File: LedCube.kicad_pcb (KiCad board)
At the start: 2 copper layers, 102 x 102 mm, 37 parts, among them J12 B10B-PHDSS-B_LF__SN_, J13 B10B-PHDSS-B_LF__SN_, J14 B10B-PHDSS-B_LF__SN_, J15 B10B-PHDSS-B_LF__SN_, J16 B10B-PHDSS-B_LF__SN_, J17 B10B-PHDSS-B_LF__SN_, J18 B10B-PHDSS-B_LF__SN_, J19 B10B-PHDSS-B_LF__SN_, J20 B10B-PHDSS-B_LF__SN_, J21 B10B-PHDSS-B_LF__SN_, U1 STM32H743VGTx, U10 SN74LVC373ARGYR, U11 SN74LVC373ARGYR, U12 SN74LVC373ARGYR, U13 SN74LVC373ARGYR, U14 SN74LVC373ARGYR, U2 SN74LVC373ARGYR, U3 SN74LVC373ARGYR, U4 SN74LVC373ARGYR, U5 SN74LVC373ARGYR, U6 SN74LVC373ARGYR, U7 SN74LVC373ARGYR, U8 SN74LVC373ARGYR, U9 SN74LVC373ARGYR

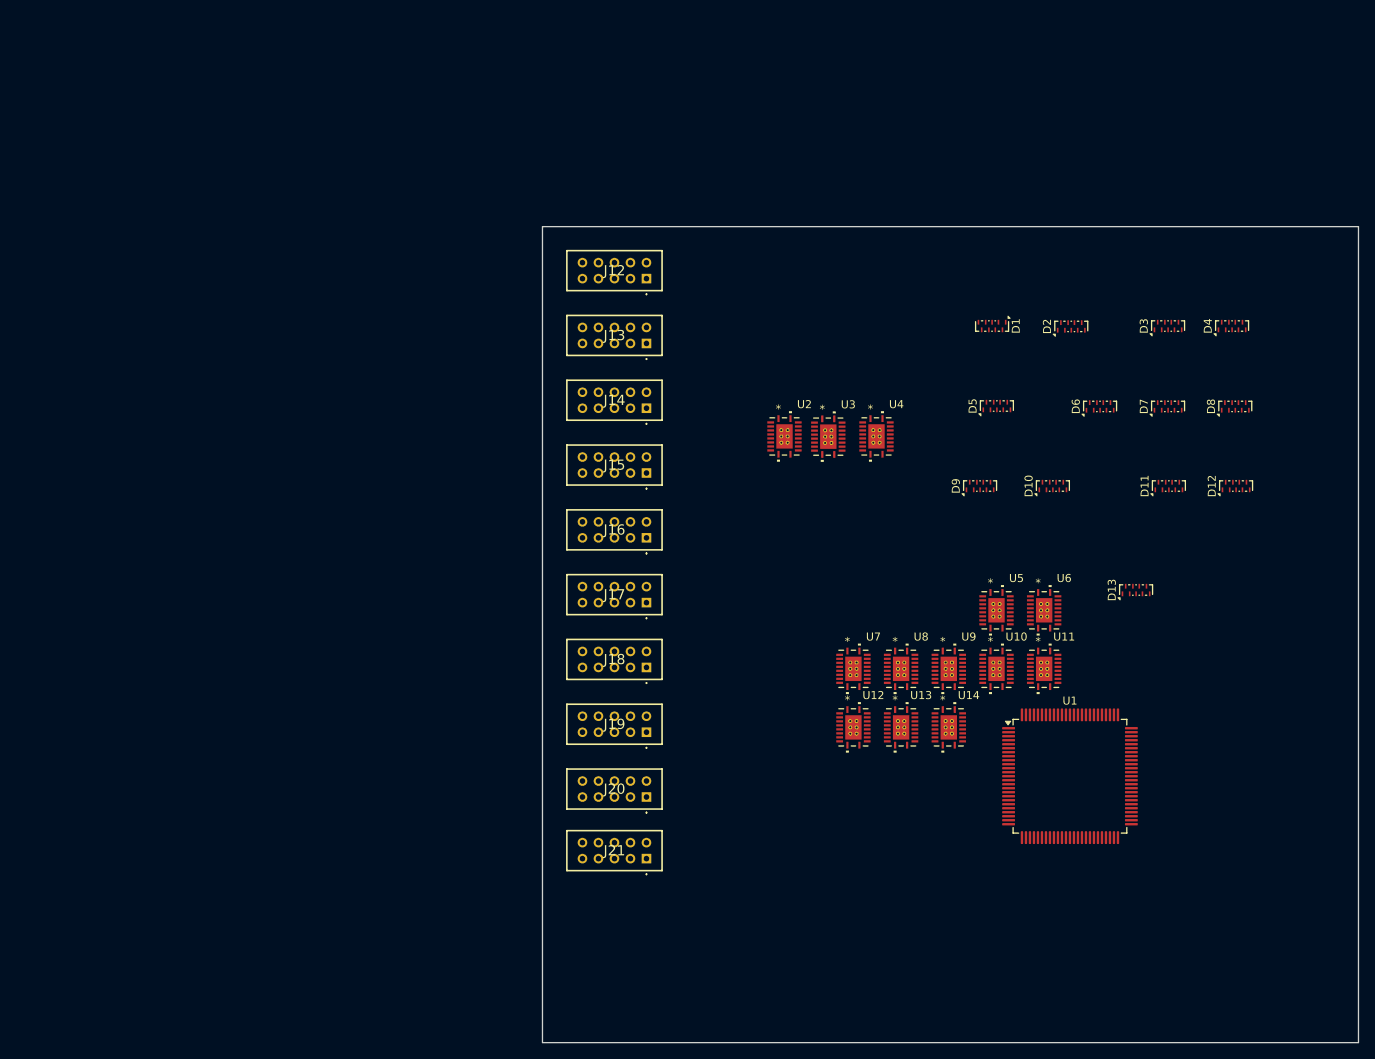
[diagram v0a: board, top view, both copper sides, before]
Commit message: Schematic + PCB
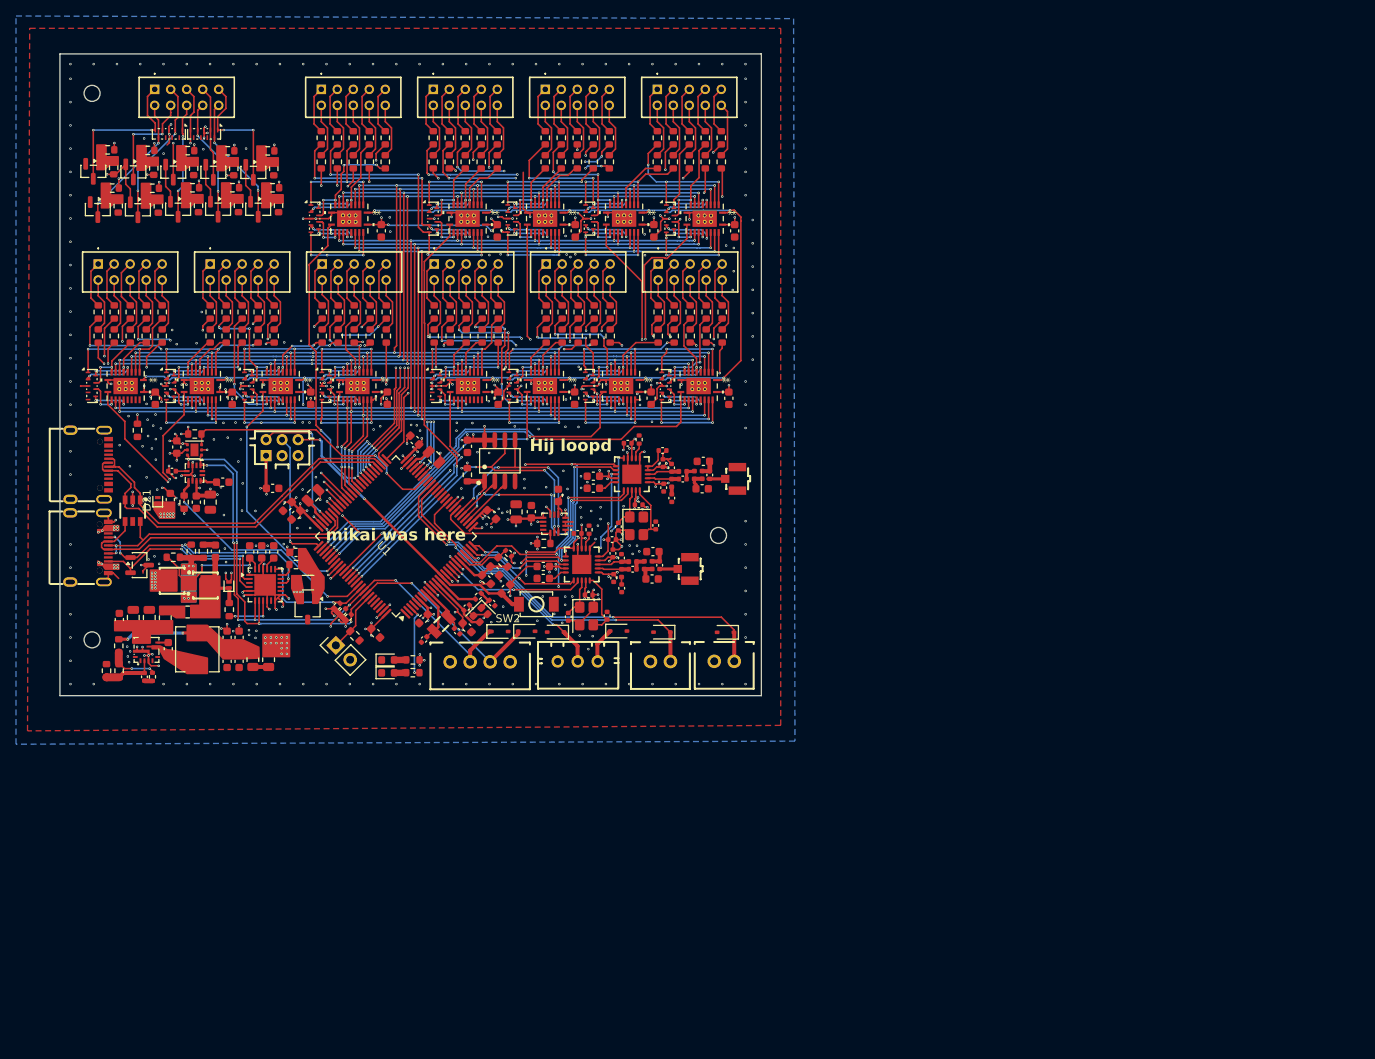
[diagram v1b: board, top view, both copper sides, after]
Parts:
- removed J12, J13, J14, J15, J16, J17, J18, J19, J20, J21: B10B-PHDSS-B_LF__SN_, JST B10B-PHDSS-B(LF)(SN):B10BPHDSSBLFSN
- added C1: 100nF, Capacitor_SMD:C_0603_1608Metric, F.Cu at (89.4, 100.8)
- added C10: 100nF, Capacitor_SMD:C_0603_1608Metric, F.Cu at (84.6, 105.6)
- added C11: 2.2uF, < 100mΩ, Capacitor_SMD:C_0805_2012Metric, F.Cu at (80.4, 84.3)
- added C12: 100nF, Capacitor_SMD:C_0603_1608Metric, F.Cu at (79.1, 104.5)
- added C13: 2.2uF, < 100mΩ, Capacitor_SMD:C_0805_2012Metric, F.Cu at (65.3, 89.1)
- added C14: 4.7uF, Capacitor_SMD:C_0603_1608Metric, F.Cu at (62.1, 90.5)
- added C17: 15pF, Capacitor_SMD:C_0402_1005Metric, F.Cu at (79.2, 107.1)
- added C18: 15pF, Capacitor_SMD:C_0402_1005Metric, F.Cu at (83.3, 106.1)
- added C19: 100nF, Capacitor_SMD:C_0603_1608Metric, F.Cu at (84.6, 83.0)
- added C2: 1uF, Capacitor_SMD:C_0603_1608Metric, F.Cu at (87.0, 99.6)
- added C20: 100nF, Capacitor_SMD:C_0603_1608Metric, F.Cu at (60.3, 88.2)
- added C21: 10uF, Capacitor_SMD:C_0805_2012Metric, F.Cu at (44.9, 104.4)
- added C22: 10uF, Capacitor_SMD:C_0805_2012Metric, F.Cu at (42.9, 104.4)
- added C23: 100nF, Capacitor_SMD:C_0603_1608Metric, F.Cu at (41.1, 104.6)
- added C24: 100nF, Capacitor_SMD:C_0603_1608Metric, F.Cu at (47.2, 108.3)
- added C25: 100pF, Capacitor_SMD:C_0402_1005Metric, F.Cu at (44.2, 111.8)
- added C26: 22uF, Capacitor_SMD:C_0603_1608Metric, F.Cu at (54.6, 106.8)
- added C27: 22uF, Capacitor_SMD:C_0603_1608Metric, F.Cu at (56.1, 106.8)
- added C28: 22uF, Capacitor_SMD:C_0603_1608Metric, F.Cu at (54.6, 109.8)
- added C29: 100nF, Capacitor_SMD:C_0603_1608Metric, F.Cu at (56.1, 109.8)
- added C3: 100nF, Capacitor_SMD:C_0603_1608Metric, F.Cu at (88.0, 98.5)
- added C30: 100nF, Capacitor_SMD:C_0603_1608Metric, F.Cu at (117.3, 77.0)
- added C31: 100nF, Capacitor_SMD:C_0603_1608Metric, F.Cu at (74.6, 76.9)
- added C32: 100nF, Capacitor_SMD:C_0603_1608Metric, F.Cu at (118.0, 56.0)
- added C33: 100nF, Capacitor_SMD:C_0603_1608Metric, F.Cu at (107.6, 76.9)
- added C34: 100nF, Capacitor_SMD:C_0603_1608Metric, F.Cu at (65.0, 76.9)
- added C35: 100nF, Capacitor_SMD:C_0603_1608Metric, F.Cu at (107.9, 56.0)
- added C36: 100nF, Capacitor_SMD:C_0603_1608Metric, F.Cu at (98.0, 76.9)
- added C37: 100nF, Capacitor_SMD:C_0603_1608Metric, F.Cu at (55.2, 77.0)
- added C38: 100nF, Capacitor_SMD:C_0603_1608Metric, F.Cu at (98.1, 56.0)
- added C39: 100nF, Capacitor_SMD:C_0603_1608Metric, F.Cu at (88.5, 77.0)
- added C4: 100nF, Capacitor_SMD:C_0603_1608Metric, F.Cu at (87.6, 91.5)
- added C40: 100nF, Capacitor_SMD:C_0603_1608Metric, F.Cu at (45.6, 77.0)
- added C41: 100nF, Capacitor_SMD:C_0603_1608Metric, F.Cu at (88.4, 56.0)
- added C42: 100nF, Capacitor_SMD:C_0603_1608Metric, F.Cu at (73.8, 56.0)
- added C43: 4.7uF, Capacitor_SMD:C_0603_1608Metric, F.Cu at (47.5, 89.6)
- added C44: 1uF, Capacitor_SMD:C_0603_1608Metric, F.Cu at (63.2, 96.2)
- added C45: 1uF, Capacitor_SMD:C_0603_1608Metric, F.Cu at (57.4, 96.2)
- added C46: 1uF, Capacitor_SMD:C_0603_1608Metric, F.Cu at (60.4, 96.2)
- added C47: 1uF, Capacitor_SMD:C_0603_1608Metric, F.Cu at (58.9, 96.2)
- added C48: 100nF, Capacitor_SMD:C_0603_1608Metric, F.Cu at (53.1, 96.1)
- added C49: 100nF, Capacitor_SMD:C_0603_1608Metric, F.Cu at (96.0, 89.1)
- added C5: 100nF, Capacitor_SMD:C_0603_1608Metric, F.Cu at (78.0, 82.2)
- added C50: 220nF, Capacitor_SMD:C_0402_1005Metric, F.Cu at (47.7, 86.1)
- added C51: 100nF, Capacitor_SMD:C_0603_1608Metric, F.Cu at (92.6, 91.1)
- added C52: 10uF, Capacitor_SMD:C_0805_2012Metric, F.Cu at (90.7, 91.2)
- added C53: 100nF, Capacitor_SMD:C_0603_1608Metric, F.Cu at (50.7, 89.9)
- added C54: 10uF, Capacitor_SMD:C_0805_2012Metric, F.Cu at (52.5, 89.9)
- added C55: 100nF, Capacitor_SMD:C_0603_1608Metric, F.Cu at (54.0, 87.4)
- added C56: 100nF, Capacitor_SMD:C_0603_1608Metric, F.Cu at (100.4, 86.7)
- added C57: 100nF, Capacitor_SMD:C_0603_1608Metric, F.Cu at (94.1, 98.0)
- added C58: 100nF, Capacitor_SMD:C_0603_1608Metric, F.Cu at (100.4, 88.2)
- added C59: 100nF, Capacitor_SMD:C_0603_1608Metric, F.Cu at (94.1, 99.5)
- added C6: 12pF, Capacitor_SMD:C_0402_1005Metric, F.Cu at (84.5, 103.1)
- added C60: 12pF, Capacitor_SMD:C_0402_1005Metric, F.Cu at (103.5, 93.0)
- added C61: 12pF, Capacitor_SMD:C_0402_1005Metric, F.Cu at (97.2, 104.3)
- added C62: 220pF, Capacitor_SMD:C_0402_1005Metric, F.Cu at (104.7, 82.6)
- added C63: 220pF, Capacitor_SMD:C_0402_1005Metric, F.Cu at (98.4, 93.8)
- added C64: 15pF, Capacitor_SMD:C_0402_1005Metric, F.Cu at (108.2, 92.8)
- added C65: 15pF, Capacitor_SMD:C_0402_1005Metric, F.Cu at (102.1, 104.1)
- added C66: 10nF, Capacitor_SMD:C_0402_1005Metric, F.Cu at (106.0, 90.3)
- added C67: 10nF, Capacitor_SMD:C_0402_1005Metric, F.Cu at (99.8, 101.5)
- added C68: 220pF, Capacitor_SMD:C_0402_1005Metric, F.Cu at (109.2, 88.1)
- added C69: 10nF, Capacitor_SMD:C_0402_1005Metric, F.Cu at (109.1, 85.1)
- added C7: 12pF, Capacitor_SMD:C_0402_1005Metric, F.Cu at (87.7, 102.5)
- added C70: 220pF, Capacitor_SMD:C_0402_1005Metric, F.Cu at (102.9, 99.4)
- added C71: 10nF, Capacitor_SMD:C_0402_1005Metric, F.Cu at (102.8, 96.3)
- added C72: 220pF, Capacitor_SMD:C_0402_1005Metric, F.Cu at (109.0, 83.5)
- added C73: 220pF, Capacitor_SMD:C_0402_1005Metric, F.Cu at (102.7, 94.6)
- added C74: 3.9pF, Capacitor_SMD:C_0402_1005Metric, F.Cu at (110.1, 85.6)
- added C75: 220pF, Capacitor_SMD:C_0402_1005Metric, F.Cu at (110.2, 89.4)
- added C76: 3.9pF, Capacitor_SMD:C_0402_1005Metric, F.Cu at (111.5, 87.0)
- added C77: 3.9pF, Capacitor_SMD:C_0402_1005Metric, F.Cu at (103.9, 96.9)
- added C78: 220pF, Capacitor_SMD:C_0402_1005Metric, F.Cu at (103.9, 100.7)
- added C79: 3.9pF, Capacitor_SMD:C_0402_1005Metric, F.Cu at (105.3, 98.3)
- added C8: 100nF, Capacitor_SMD:C_0603_1608Metric, F.Cu at (63.2, 91.5)
- added C80: 8.2pF, Capacitor_SMD:C_0603_1608Metric, F.Cu at (114.0, 88.3)
- added C81: 8.2pF, Capacitor_SMD:C_0603_1608Metric, F.Cu at (107.7, 99.5)
- added C82: 5.6pF, Capacitor_SMD:C_0603_1608Metric, F.Cu at (114.1, 84.8)
- added C83: 220pF, Capacitor_SMD:C_0402_1005Metric, F.Cu at (114.9, 86.5)
- added C84: 5.6pF, Capacitor_SMD:C_0603_1608Metric, F.Cu at (107.8, 96.1)
- added C85: 220pF, Capacitor_SMD:C_0402_1005Metric, F.Cu at (108.7, 97.8)
- added C86: 100nF, Capacitor_SMD:C_0603_1608Metric, F.Cu at (48.3, 83.0)
- added C9: 100nF, Capacitor_SMD:C_0603_1608Metric, F.Cu at (73.1, 106.3)
- added CN1: B2B-XH-A (LF)(SN), easyeda2kicad:CONN-TH_B2B-XH-A-LF-SN, F.Cu at (116.7, 109.8)
- added CN2: B2B-XH-A (LF)(SN), easyeda2kicad:CONN-TH_B2B-XH-A-LF-SN, F.Cu at (108.7, 109.9)
- added D14: SP7538P, Package_DFN_QFN:UDFN-9_1.0x3.8mm_P0.5mm, F.Cu at (80.7, 75.4)
- added D15: SP7538P, Package_DFN_QFN:UDFN-9_1.0x3.8mm_P0.5mm, F.Cu at (37.7, 75.4)
- added D16: SP7538P, Package_DFN_QFN:UDFN-9_1.0x3.8mm_P0.5mm, F.Cu at (80.3, 54.5)
- added D17: SP7538P, Package_DFN_QFN:UDFN-9_1.0x3.8mm_P0.5mm, F.Cu at (65.5, 54.5)
- added D18: SP7538P, Package_DFN_QFN:UDFN-9_1.0x3.8mm_P0.5mm, F.Cu at (51.7, 43.9)
- added D19: SP7538P, Package_DFN_QFN:UDFN-9_1.0x3.8mm_P0.5mm, F.Cu at (47.3, 43.9)
- added D20: PRTR5V0U4D, easyeda2kicad:SOT-23-6_L2.9-W1.6-P0.95-LS2.8-BR, F.Cu at (42.8, 91.0)
- added D21: ESDA25P35-1U1M, Diode_SMD:D_SOD-882, F.Cu at (45.9, 89.7)
- added D22: ESDA25L, Package_TO_SOT_SMD:SOT-23-3, F.Cu at (43.6, 97.8)
- added D23: BAT54, Package_TO_SOT_SMD:TSOT-23, F.Cu at (64.7, 103.3)
- added D24: ESDA25P35-1U1M, Diode_SMD:D_SOD-882, F.Cu at (54.8, 100.3)
- added D25: PESD3V3L1BA, Diode_SMD:D_SOD-323, F.Cu at (88.7, 106.1)
- added D26: PESD3V3L1BA, Diode_SMD:D_SOD-323, F.Cu at (92.0, 106.1)
- added D27: PESD3V3L1BA, Diode_SMD:D_SOD-323, F.Cu at (116.9, 106.2)
- added D28: PESD3V3L1BA, Diode_SMD:D_SOD-323, F.Cu at (108.9, 106.2)
- added FB1: FerriteBead, Resistor_SMD:R_0402_1005Metric, F.Cu at (89.8, 96.3)
- added FB2: FerriteBead, Resistor_SMD:R_0805_2012Metric, F.Cu at (46.9, 104.4)
- added FB3: FerriteBead, Resistor_SMD:R_0805_2012Metric, F.Cu at (57.8, 109.6)
- added J1: B10B-PHDSS-B_LF__SN_, JST B10B-PHDSS-B(LF)(SN):B10BPHDSSBLFSN, F.Cu at (108.5, 60.2)
- added J10: B10B-PHDSS-B_LF__SN_, JST B10B-PHDSS-B(LF)(SN):B10BPHDSSBLFSN, F.Cu at (66.4, 38.3)
- added J11: B10B-PHDSS-B_LF__SN_, JST B10B-PHDSS-B(LF)(SN):B10BPHDSSBLFSN, F.Cu at (45.5, 38.3)
- added J2: B10B-PHDSS-B_LF__SN_, JST B10B-PHDSS-B(LF)(SN):B10BPHDSSBLFSN, F.Cu at (66.5, 60.2)
- added J3: B10B-PHDSS-B_LF__SN_, JST B10B-PHDSS-B(LF)(SN):B10BPHDSSBLFSN, F.Cu at (108.4, 38.3)
- added J4: B10B-PHDSS-B_LF__SN_, JST B10B-PHDSS-B(LF)(SN):B10BPHDSSBLFSN, F.Cu at (94.5, 60.2)
- added J5: B10B-PHDSS-B_LF__SN_, JST B10B-PHDSS-B(LF)(SN):B10BPHDSSBLFSN, F.Cu at (52.5, 60.2)
- added J6: B10B-PHDSS-B_LF__SN_, JST B10B-PHDSS-B(LF)(SN):B10BPHDSSBLFSN, F.Cu at (94.4, 38.3)
- added J7: B10B-PHDSS-B_LF__SN_, JST B10B-PHDSS-B(LF)(SN):B10BPHDSSBLFSN, F.Cu at (80.5, 60.2)
- added J8: B10B-PHDSS-B_LF__SN_, JST B10B-PHDSS-B(LF)(SN):B10BPHDSSBLFSN, F.Cu at (38.5, 60.2)
- added J9: B10B-PHDSS-B_LF__SN_, JST B10B-PHDSS-B(LF)(SN):B10BPHDSSBLFSN, F.Cu at (80.4, 38.3)
- added JP1: Jumper_2_Bridged, Resistor_SMD:R_0805_2012Metric, F.Cu at (49.6, 103.7)
- added JP2: Jumper_2_Bridged, Resistor_SMD:R_0805_2012Metric, F.Cu at (59.8, 109.6)
- added JP3: Jumper_2_Open, Connector_PinHeader_2.54mm:PinHeader_1x02_P2.54mm_Vertical, F.Cu at (68.2, 107.8)
- added JP4: U.FL-R-SMT-1(80), easyeda2kicad:RF-SMD_FRF05002-JSS103M, F.Cu at (117.6, 87.0)
- added JP5: U.FL-R-SMT-1(80), easyeda2kicad:RF-SMD_FRF05002-JSS103M, F.Cu at (111.7, 98.3)
- added L1: 2.2uH, Inductor_SMD:L_Chilisin_BMRB00050518-B, F.Cu at (50.9, 108.3)
- added L2: 27nH, Inductor_SMD:L_0402_1005Metric, F.Cu at (110.1, 87.5)
- added L3: 27nH, Inductor_SMD:L_0402_1005Metric, F.Cu at (111.5, 86.1)
- added L4: 27nH, Inductor_SMD:L_0402_1005Metric, F.Cu at (103.9, 98.8)
- added L5: 27nH, Inductor_SMD:L_0402_1005Metric, F.Cu at (105.3, 97.4)
- added L6: 22nH, Inductor_SMD:L_0402_1005Metric, F.Cu at (113.0, 86.5)
- added L7: 22nH, Inductor_SMD:L_0402_1005Metric, F.Cu at (106.7, 97.8)
- added L8: 27nH, Inductor_SMD:L_0402_1005Metric, F.Cu at (114.0, 86.5)
- added L9: 27nH, Inductor_SMD:L_0402_1005Metric, F.Cu at (107.7, 97.8)
- added Q1: AO3400A, Package_TO_SOT_SMD:SOT-23, F.Cu at (58.5, 53.3)
- added Q10: AO3400A, Package_TO_SOT_SMD:SOT-23, F.Cu at (57.9, 48.7)
- added Q11: JSM7409B, easyeda2kicad:POWERVDFN-8_L3.2-W3.1-P0.65-LS3.3-BL-1, F.Cu at (51.9, 100.4)
- added Q13: JSM7409B, easyeda2kicad:POWERVDFN-8_L3.2-W3.1-P0.65-LS3.3-BL-1, F.Cu at (47.7, 99.7)
- added Q2: AO3400A, Package_TO_SOT_SMD:SOT-23, F.Cu at (53.5, 53.3)
- added Q3: AO3400A, Package_TO_SOT_SMD:SOT-23, F.Cu at (48.5, 53.3)
- added Q4: AO3400A, Package_TO_SOT_SMD:SOT-23, F.Cu at (42.9, 48.7)
- added Q5: AO3400A, Package_TO_SOT_SMD:SOT-23, F.Cu at (38.4, 53.4)
- added Q6: AO3400A, Package_TO_SOT_SMD:SOT-23, F.Cu at (37.9, 48.6)
- added Q7: AO3400A, Package_TO_SOT_SMD:SOT-23, F.Cu at (43.4, 53.4)
- added Q8: AO3400A, Package_TO_SOT_SMD:SOT-23, F.Cu at (47.9, 48.7)
- added Q9: AO3400A, Package_TO_SOT_SMD:SOT-23, F.Cu at (52.9, 48.7)
- added R1: 10K, Resistor_SMD:R_0603_1608Metric, F.Cu at (70.6, 106.7)
- added R10: 20k, Resistor_SMD:R_0402_1005Metric, F.Cu at (45.2, 111.8)
- added R100: 47Ω, Resistor_SMD:R_0603_1608Metric, F.Cu at (88.3, 47.4)
- added R101: 47Ω, Resistor_SMD:R_0603_1608Metric, F.Cu at (86.3, 47.4)
- added R102: 47Ω, Resistor_SMD:R_0603_1608Metric, F.Cu at (84.3, 47.4)
- added R103: 47Ω, Resistor_SMD:R_0603_1608Metric, F.Cu at (82.3, 47.4)
- added R104: 47Ω, Resistor_SMD:R_0603_1608Metric, F.Cu at (80.3, 47.4)
- added R105: 47Ω, Resistor_SMD:R_0603_1608Metric, F.Cu at (74.4, 44.4)
- added R106: 47Ω, Resistor_SMD:R_0603_1608Metric, F.Cu at (72.4, 44.4)
- added R107: 47Ω, Resistor_SMD:R_0603_1608Metric, F.Cu at (70.4, 44.4)
- added R108: 47Ω, Resistor_SMD:R_0603_1608Metric, F.Cu at (68.4, 44.4)
- added R109: 47Ω, Resistor_SMD:R_0603_1608Metric, F.Cu at (66.4, 44.4)
- added R11: 49.9, Resistor_SMD:R_0603_1608Metric, F.Cu at (41.0, 107.9)
- added R110: 47Ω, Resistor_SMD:R_0603_1608Metric, F.Cu at (74.3, 47.4)
- added R111: 47Ω, Resistor_SMD:R_0603_1608Metric, F.Cu at (72.3, 47.4)
- added R112: 47Ω, Resistor_SMD:R_0603_1608Metric, F.Cu at (70.3, 47.4)
- added R113: 47Ω, Resistor_SMD:R_0603_1608Metric, F.Cu at (68.3, 47.4)
- added R114: 47Ω, Resistor_SMD:R_0603_1608Metric, F.Cu at (66.3, 47.4)
- added R115: 1k, Resistor_SMD:R_0603_1608Metric, F.Cu at (59.7, 46.0)
- added R116: 1k, Resistor_SMD:R_0603_1608Metric, F.Cu at (54.7, 46.0)
- added R117: 1k, Resistor_SMD:R_0603_1608Metric, F.Cu at (49.6, 46.0)
- added R118: 1k, Resistor_SMD:R_0603_1608Metric, F.Cu at (45.2, 50.7)
- added R119: 1k, Resistor_SMD:R_0603_1608Metric, F.Cu at (39.7, 45.9)
- added R12: 45.3k, Resistor_SMD:R_0603_1608Metric, F.Cu at (41.1, 111.0)
- added R120: 1k, Resistor_SMD:R_0603_1608Metric, F.Cu at (40.2, 50.7)
- added R121: 1k, Resistor_SMD:R_0603_1608Metric, F.Cu at (44.7, 46.0)
- added R122: 1k, Resistor_SMD:R_0603_1608Metric, F.Cu at (50.2, 50.6)
- added R123: 1k, Resistor_SMD:R_0603_1608Metric, F.Cu at (60.3, 50.6)
- added R124: 1k, Resistor_SMD:R_0603_1608Metric, F.Cu at (55.2, 50.6)
- added R125: 100K, Resistor_SMD:R_0603_1608Metric, F.Cu at (61.0, 52.9)
- added R126: 100K, Resistor_SMD:R_0603_1608Metric, F.Cu at (56.0, 52.9)
- added R127: 100K, Resistor_SMD:R_0603_1608Metric, F.Cu at (51.0, 52.9)
- added R128: 100K, Resistor_SMD:R_0603_1608Metric, F.Cu at (45.4, 48.2)
- added R129: 100K, Resistor_SMD:R_0603_1608Metric, F.Cu at (41.0, 52.9)
- added R13: 10K, Resistor_SMD:R_0603_1608Metric, F.Cu at (39.5, 111.0)
- added R130: 100K, Resistor_SMD:R_0603_1608Metric, F.Cu at (40.4, 48.1)
- added R131: 100K, Resistor_SMD:R_0603_1608Metric, F.Cu at (46.0, 52.9)
- added R132: 100K, Resistor_SMD:R_0603_1608Metric, F.Cu at (50.4, 48.2)
- added R133: 100K, Resistor_SMD:R_0603_1608Metric, F.Cu at (55.4, 48.3)
- added R134: 100K, Resistor_SMD:R_0603_1608Metric, F.Cu at (60.4, 48.3)
- added R135: 470, Resistor_SMD:R_1206_3216Metric, F.Cu at (64.7, 100.0)
- added R136: 1k, Resistor_SMD:R_0603_1608Metric, F.Cu at (63.2, 97.7)
- added R137: 22k, Resistor_SMD:R_0603_1608Metric, F.Cu at (50.1, 96.1)
- added R138: 1k, Resistor_SMD:R_0603_1608Metric, F.Cu at (54.9, 103.4)
- added R139: 100K, Resistor_SMD:R_0603_1608Metric, F.Cu at (47.9, 96.8)
- added R14: 10K, Resistor_SMD:R_0603_1608Metric, F.Cu at (43.4, 81.0)
- added R140: 100, Resistor_SMD:R_0603_1608Metric, F.Cu at (51.6, 96.1)
- added R141: 10K, Resistor_SMD:R_0603_1608Metric, F.Cu at (50.5, 81.4)
- added R142: 10K, Resistor_SMD:R_0603_1608Metric, F.Cu at (94.2, 95.1)
- added R143: 10K, Resistor_SMD:R_0603_1608Metric, F.Cu at (49.2, 89.9)
- added R144: 56K, Resistor_SMD:R_0402_1005Metric, F.Cu at (106.1, 82.1)
- added R145: 56K, Resistor_SMD:R_0402_1005Metric, F.Cu at (99.8, 93.4)
- added R15: 47Ω, Resistor_SMD:R_0603_1608Metric, F.Cu at (116.5, 66.2)
- added R16: 47Ω, Resistor_SMD:R_0603_1608Metric, F.Cu at (114.5, 66.2)
- added R17: 47Ω, Resistor_SMD:R_0603_1608Metric, F.Cu at (112.5, 66.2)
- added R18: 47Ω, Resistor_SMD:R_0603_1608Metric, F.Cu at (110.5, 66.2)
- added R19: 47Ω, Resistor_SMD:R_0603_1608Metric, F.Cu at (108.5, 66.2)
- added R2: 47Ω, Resistor_SMD:R_0603_1608Metric, F.Cu at (89.1, 97.4)
- added R20: 47Ω, Resistor_SMD:R_0603_1608Metric, F.Cu at (102.5, 66.2)
- added R21: 47Ω, Resistor_SMD:R_0603_1608Metric, F.Cu at (100.5, 66.2)
- added R22: 47Ω, Resistor_SMD:R_0603_1608Metric, F.Cu at (98.5, 66.2)
- added R23: 47Ω, Resistor_SMD:R_0603_1608Metric, F.Cu at (96.5, 66.2)
- added R24: 47Ω, Resistor_SMD:R_0603_1608Metric, F.Cu at (94.5, 66.2)
- added R25: 47Ω, Resistor_SMD:R_0603_1608Metric, F.Cu at (102.5, 69.2)
- added R26: 47Ω, Resistor_SMD:R_0603_1608Metric, F.Cu at (100.5, 69.2)
- added R27: 47Ω, Resistor_SMD:R_0603_1608Metric, F.Cu at (98.5, 69.2)
- added R28: 47Ω, Resistor_SMD:R_0603_1608Metric, F.Cu at (96.5, 69.2)
- added R29: 47Ω, Resistor_SMD:R_0603_1608Metric, F.Cu at (94.5, 69.2)
- added R3: 220, Resistor_SMD:R_0603_1608Metric, F.Cu at (77.8, 109.7)
- added R30: 47Ω, Resistor_SMD:R_0603_1608Metric, F.Cu at (116.5, 69.2)
- added R31: 47Ω, Resistor_SMD:R_0603_1608Metric, F.Cu at (114.5, 69.2)
- added R32: 47Ω, Resistor_SMD:R_0603_1608Metric, F.Cu at (112.5, 69.2)
- added R33: 47Ω, Resistor_SMD:R_0603_1608Metric, F.Cu at (110.5, 69.2)
- added R34: 47Ω, Resistor_SMD:R_0603_1608Metric, F.Cu at (108.5, 69.2)
- added R35: 47Ω, Resistor_SMD:R_0603_1608Metric, F.Cu at (88.5, 66.2)
- added R36: 47Ω, Resistor_SMD:R_0603_1608Metric, F.Cu at (86.5, 66.2)
- added R37: 47Ω, Resistor_SMD:R_0603_1608Metric, F.Cu at (84.5, 66.2)
- added R38: 47Ω, Resistor_SMD:R_0603_1608Metric, F.Cu at (82.5, 66.2)
- added R39: 47Ω, Resistor_SMD:R_0603_1608Metric, F.Cu at (80.5, 66.2)
- added R4: 22, Resistor_SMD:R_0402_1005Metric, F.Cu at (86.0, 101.7)
- added R40: 47Ω, Resistor_SMD:R_0603_1608Metric, F.Cu at (88.5, 69.2)
- added R41: 47Ω, Resistor_SMD:R_0603_1608Metric, F.Cu at (86.5, 69.2)
- added R42: 47Ω, Resistor_SMD:R_0603_1608Metric, F.Cu at (84.5, 69.2)
- added R43: 47Ω, Resistor_SMD:R_0603_1608Metric, F.Cu at (82.5, 69.2)
- added R44: 47Ω, Resistor_SMD:R_0603_1608Metric, F.Cu at (80.5, 69.2)
- added R45: 47Ω, Resistor_SMD:R_0603_1608Metric, F.Cu at (74.5, 66.2)
- added R46: 47Ω, Resistor_SMD:R_0603_1608Metric, F.Cu at (72.5, 66.2)
- added R47: 47Ω, Resistor_SMD:R_0603_1608Metric, F.Cu at (70.5, 66.2)
- added R48: 47Ω, Resistor_SMD:R_0603_1608Metric, F.Cu at (68.5, 66.2)
- added R49: 47Ω, Resistor_SMD:R_0603_1608Metric, F.Cu at (66.5, 66.2)
- added R5: 220, Resistor_SMD:R_0603_1608Metric, F.Cu at (77.8, 111.3)
- added R50: 47Ω, Resistor_SMD:R_0603_1608Metric, F.Cu at (74.5, 69.2)
- added R51: 47Ω, Resistor_SMD:R_0603_1608Metric, F.Cu at (72.5, 69.2)
- added R52: 47Ω, Resistor_SMD:R_0603_1608Metric, F.Cu at (70.5, 69.2)
- added R53: 47Ω, Resistor_SMD:R_0603_1608Metric, F.Cu at (68.5, 69.2)
- added R54: 47Ω, Resistor_SMD:R_0603_1608Metric, F.Cu at (66.5, 69.2)
- added R55: 47Ω, Resistor_SMD:R_0603_1608Metric, F.Cu at (60.5, 66.2)
- added R56: 47Ω, Resistor_SMD:R_0603_1608Metric, F.Cu at (58.5, 66.2)
- added R57: 47Ω, Resistor_SMD:R_0603_1608Metric, F.Cu at (56.5, 66.2)
- added R58: 47Ω, Resistor_SMD:R_0603_1608Metric, F.Cu at (54.5, 66.2)
- added R59: 47Ω, Resistor_SMD:R_0603_1608Metric, F.Cu at (52.5, 66.2)
- added R6: 2.2K, Resistor_SMD:R_0402_1005Metric, F.Cu at (69.7, 104.3)
- added R60: 47Ω, Resistor_SMD:R_0603_1608Metric, F.Cu at (60.5, 69.2)
- added R61: 47Ω, Resistor_SMD:R_0603_1608Metric, F.Cu at (58.5, 69.2)
- added R62: 47Ω, Resistor_SMD:R_0603_1608Metric, F.Cu at (56.5, 69.2)
- added R63: 47Ω, Resistor_SMD:R_0603_1608Metric, F.Cu at (54.5, 69.2)
- added R64: 47Ω, Resistor_SMD:R_0603_1608Metric, F.Cu at (52.5, 69.2)
- added R65: 47Ω, Resistor_SMD:R_0603_1608Metric, F.Cu at (46.5, 66.2)
- added R66: 47Ω, Resistor_SMD:R_0603_1608Metric, F.Cu at (44.5, 66.2)
- added R67: 47Ω, Resistor_SMD:R_0603_1608Metric, F.Cu at (42.5, 66.2)
- added R68: 47Ω, Resistor_SMD:R_0603_1608Metric, F.Cu at (40.5, 66.2)
- added R69: 47Ω, Resistor_SMD:R_0603_1608Metric, F.Cu at (38.5, 66.2)
- added R7: 2.2K, Resistor_SMD:R_0402_1005Metric, F.Cu at (69.0, 103.6)
- added R70: 47Ω, Resistor_SMD:R_0603_1608Metric, F.Cu at (46.5, 69.2)
- added R71: 47Ω, Resistor_SMD:R_0603_1608Metric, F.Cu at (44.5, 69.2)
- added R72: 47Ω, Resistor_SMD:R_0603_1608Metric, F.Cu at (42.5, 69.2)
- added R73: 47Ω, Resistor_SMD:R_0603_1608Metric, F.Cu at (40.5, 69.2)
- added R74: 47Ω, Resistor_SMD:R_0603_1608Metric, F.Cu at (38.5, 69.2)
- added R75: 47Ω, Resistor_SMD:R_0603_1608Metric, F.Cu at (116.4, 44.4)
- added R76: 47Ω, Resistor_SMD:R_0603_1608Metric, F.Cu at (114.4, 44.4)
- added R77: 47Ω, Resistor_SMD:R_0603_1608Metric, F.Cu at (112.4, 44.4)
- added R78: 47Ω, Resistor_SMD:R_0603_1608Metric, F.Cu at (110.4, 44.4)
- added R79: 47Ω, Resistor_SMD:R_0603_1608Metric, F.Cu at (108.4, 44.4)
- added R8: 10K, Resistor_SMD:R_0603_1608Metric, F.Cu at (84.6, 86.5)
- added R80: 47Ω, Resistor_SMD:R_0603_1608Metric, F.Cu at (116.3, 47.4)
- added R81: 47Ω, Resistor_SMD:R_0603_1608Metric, F.Cu at (114.3, 47.4)
- added R82: 47Ω, Resistor_SMD:R_0603_1608Metric, F.Cu at (112.3, 47.4)
- added R83: 47Ω, Resistor_SMD:R_0603_1608Metric, F.Cu at (110.3, 47.4)
- added R84: 47Ω, Resistor_SMD:R_0603_1608Metric, F.Cu at (108.4, 47.4)
- added R85: 47Ω, Resistor_SMD:R_0603_1608Metric, F.Cu at (102.4, 44.4)
- added R86: 47Ω, Resistor_SMD:R_0603_1608Metric, F.Cu at (100.4, 44.4)
- added R87: 47Ω, Resistor_SMD:R_0603_1608Metric, F.Cu at (98.4, 44.4)
- added R88: 47Ω, Resistor_SMD:R_0603_1608Metric, F.Cu at (96.4, 44.4)
- added R89: 47Ω, Resistor_SMD:R_0603_1608Metric, F.Cu at (94.4, 44.4)
- added R9: 2.2K, Resistor_SMD:R_0402_1005Metric, F.Cu at (68.3, 102.9)
- added R90: 47Ω, Resistor_SMD:R_0603_1608Metric, F.Cu at (102.3, 47.4)
- added R91: 47Ω, Resistor_SMD:R_0603_1608Metric, F.Cu at (100.3, 47.4)
- added R92: 47Ω, Resistor_SMD:R_0603_1608Metric, F.Cu at (98.3, 47.4)
- added R93: 47Ω, Resistor_SMD:R_0603_1608Metric, F.Cu at (96.3, 47.4)
- added R94: 47Ω, Resistor_SMD:R_0603_1608Metric, F.Cu at (94.3, 47.4)
- added R95: 47Ω, Resistor_SMD:R_0603_1608Metric, F.Cu at (88.4, 44.4)
- added R96: 47Ω, Resistor_SMD:R_0603_1608Metric, F.Cu at (86.4, 44.4)
- added R97: 47Ω, Resistor_SMD:R_0603_1608Metric, F.Cu at (84.4, 44.4)
- added R98: 47Ω, Resistor_SMD:R_0603_1608Metric, F.Cu at (82.4, 44.4)
- added R99: 47Ω, Resistor_SMD:R_0603_1608Metric, F.Cu at (80.4, 44.4)
- added REF**: MountingHole_2mm, MountingHole:MountingHole_2mm, F.Cu at (116.0, 94.1)
- added REF**: MountingHole_2mm, MountingHole:MountingHole_2mm, F.Cu at (37.7, 38.8)
- added REF**: MountingHole_2mm, MountingHole:MountingHole_2mm, F.Cu at (37.7, 107.2)
- added SW2: TS-1088-AR02016, easyeda2kicad:SW-SMD_L3.9-W3.0-P4.45, F.Cu at (93.2, 102.7)
- added U15: SN74LVC373ARGYR, SN74LVC373ARGYR:RGY20_3P05X2P05, F.Cu at (94.3, 54.5)
- added U16: SN74LVC373ARGYR, SN74LVC373ARGYR:RGY20_3P05X2P05, F.Cu at (84.7, 75.4)
- added U17: SN74LVC373ARGYR, SN74LVC373ARGYR:RGY20_3P05X2P05, F.Cu at (41.9, 75.4)
- added U18: SN74LVC373ARGYR, SN74LVC373ARGYR:RGY20_3P05X2P05, F.Cu at (84.6, 54.5)
- added U19: SN74LVC373ARGYR, SN74LVC373ARGYR:RGY20_3P05X2P05, F.Cu at (69.9, 54.5)
- added U20: STUSB4500QTR, Package_DFN_QFN:QFN-24-1EP_4x4mm_P0.5mm_EP2.7x2.7mm, F.Cu at (59.3, 100.3)
- added U21: ASM330LHBG1TR, easyeda2kicad:LGA-14_L3.0-W2.5-P0.50-BL, F.Cu at (95.5, 92.6)
- added U22: IIS2MDCTR, easyeda2kicad:LGA-12_L2.0-W2.0-P0.50-TL, F.Cu at (50.5, 86.3)
- added U23: TMP117xxDRV, Package_SON:WSON-6-1EP_2x2mm_P0.65mm_EP1x1.6mm, F.Cu at (50.5, 83.4)
- added U24: CC1101RGPR, easyeda2kicad:QFN-20_L4.0-W4.0-P0.5-TL-EP, F.Cu at (105.2, 86.5)
- added U25: CC1101RGPR, easyeda2kicad:QFN-20_L4.0-W4.0-P0.5-TL-EP, F.Cu at (98.9, 97.7)
- added USB1: TYPE-C 16PIN 2MD(073), easyeda2kicad:USB-C-SMD_TYPE-C-6PIN-2MD-073, F.Cu at (37.4, 95.6)
- added USB2: TYPE-C 16PIN 2MD(073), easyeda2kicad:USB-C-SMD_TYPE-C-6PIN-2MD-073, F.Cu at (37.4, 85.3)
- added X1: Q13FC1350000400, easyeda2kicad:FC-135R_L3.2-W1.5, F.Cu at (81.4, 105.2)
- added Y1: MDH 2.D.1.480008813, Crystal:Crystal_SMD_2016-4Pin_2.0x1.6mm, F.Cu at (86.3, 104.0)
- added Y3: Crystal_GND24, Crystal:Crystal_SMD_3225-4Pin_3.2x2.5mm, F.Cu at (105.8, 92.9)
- added Y4: Crystal_GND24, Crystal:Crystal_SMD_3225-4Pin_3.2x2.5mm, F.Cu at (99.5, 104.2)
- D1: value SP7538P -> LED_PWR; footprint Package_DFN_QFN:UDFN-9_1.0x3.8mm_P0.5mm -> LED_SMD:LED_0603_1608Metric
- D2: value SP7538P -> LED_STAT; footprint Package_DFN_QFN:UDFN-9_1.0x3.8mm_P0.5mm -> LED_SMD:LED_0603_1608Metric
- D3, D4: value SP7538P -> PESD3V3L1BA; footprint Package_DFN_QFN:UDFN-9_1.0x3.8mm_P0.5mm -> Diode_SMD:D_SOD-323
- U2: value SN74LVC373ARGYR -> M95M04-DRMN6TP; footprint SN74LVC373ARGYR:RGY20_3P05X2P05 -> easyeda2kicad:SOIC-8_L4.9-W3.9-P1.27-LS6.0-BL
- U3: value SN74LVC373ARGYR -> B3B-XH-A(LF)(SN); footprint SN74LVC373ARGYR:RGY20_3P05X2P05 -> easyeda2kicad:CONN-TH_3P-P2.50_A2501WV2-3P
- U4: value SN74LVC373ARGYR -> B4B-XH-A(LF)(SN); footprint SN74LVC373ARGYR:RGY20_3P05X2P05 -> easyeda2kicad:CONN-TH_B4B-XH-A-LF-SN
- U5: value SN74LVC373ARGYR -> HC-PHD2.0-2X3A; footprint SN74LVC373ARGYR:RGY20_3P05X2P05 -> easyeda2kicad:HDR-TH_6P-P2.00-V-F-R2-C3-S2.00-4
- U6: value SN74LVC373ARGYR -> TPS56637RPAR; footprint SN74LVC373ARGYR:RGY20_3P05X2P05 -> easyeda2kicad:VQFN-HR-10_L3.0-W3.0_RPA
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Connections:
- D1 pad 1: OUT_0_1 -> GND
- D1 pad 2: OUT_0_2 -> Net-(D1-A)
- D10 pad 1: OUT_6_9 -> Net-(D10-K1)
- D10 pad 2: OUT_6_10 -> Net-(D10-K2)
- D10 pad 4: OUT_7_1 -> Net-(D10-K3)
- D10 pad 5: OUT_7_2 -> Net-(D10-K4)
- D10 pad 6: OUT_7_3 -> Net-(D10-K5)
- D10 pad 7: OUT_7_4 -> Net-(D10-K6)
- D10 pad 8: OUT_7_5 -> Net-(D10-K7)
- D10 pad 9: OUT_7_6 -> Net-(D10-K8)
- D11 pad 1: OUT_7_7 -> Net-(D11-K1)
- D11 pad 2: OUT_7_8 -> Net-(D11-K2)
- D11 pad 4: OUT_7_9 -> Net-(D11-K3)
- D11 pad 5: OUT_7_10 -> Net-(D11-K4)
- D11 pad 6: OUT_8_1 -> Net-(D11-K5)
- D11 pad 7: OUT_8_2 -> Net-(D11-K6)
- D11 pad 8: OUT_8_3 -> Net-(D11-K7)
- D11 pad 9: OUT_8_4 -> Net-(D11-K8)
- D12 pad 1: OUT_8_5 -> Net-(D12-K1)
- D12 pad 2: OUT_8_6 -> Net-(D12-K2)
- D12 pad 4: OUT_8_7 -> Net-(D12-K3)
- D12 pad 5: OUT_8_8 -> Net-(D12-K4)
- D12 pad 6: OUT_8_9 -> Net-(D12-K5)
- D12 pad 7: OUT_8_10 -> Net-(D12-K6)
- D12 pad 8: OUT_9_9 -> Net-(D12-K7)
- D12 pad 9: OUT_9_10 -> Net-(D12-K8)
- D13 pad 1: OUT_9_1 -> Net-(D13-K1)
- D13 pad 2: OUT_9_2 -> Net-(D13-K2)
- D13 pad 4: OUT_9_3 -> Net-(D13-K3)
- D13 pad 5: OUT_9_4 -> Net-(D13-K4)
- D13 pad 6: OUT_9_5 -> Net-(D13-K5)
- D13 pad 7: OUT_9_6 -> Net-(D13-K6)
- D13 pad 8: OUT_9_7 -> Net-(D13-K7)
- D13 pad 9: OUT_9_8 -> Net-(D13-K8)
- D2 pad 1: OUT_0_9 -> GND
- D2 pad 2: OUT_0_10 -> Net-(D2-A)
- D3 pad 1: OUT_1_7 -> +3.3V
- D3 pad 2: OUT_1_8 -> GND
- D4 pad 1: OUT_2_5 -> Net-(D4-K)
- D4 pad 2: OUT_2_6 -> GND
- D5 pad 1: OUT_3_1 -> Net-(D5-K1)
- D5 pad 2: OUT_3_2 -> Net-(D5-K2)
- D5 pad 4: OUT_3_3 -> Net-(D5-K3)
- D5 pad 5: OUT_3_4 -> Net-(D5-K4)
- D5 pad 6: OUT_3_5 -> Net-(D5-K5)
- D5 pad 7: OUT_3_6 -> Net-(D5-K6)
- D5 pad 8: OUT_3_7 -> Net-(D5-K7)
- D5 pad 9: OUT_3_8 -> Net-(D5-K8)
- D6 pad 1: OUT_3_9 -> Net-(D6-K1)
- D6 pad 2: OUT_3_10 -> Net-(D6-K2)
- D6 pad 4: OUT_4_1 -> Net-(D6-K3)
- D6 pad 5: OUT_4_2 -> Net-(D6-K4)
- D6 pad 6: OUT_4_3 -> Net-(D6-K5)
- D6 pad 7: OUT_4_4 -> Net-(D6-K6)
- D6 pad 8: OUT_4_5 -> Net-(D6-K7)
- D6 pad 9: OUT_4_6 -> Net-(D6-K8)
- D7 pad 1: OUT_4_7 -> Net-(D7-K1)
- D7 pad 2: OUT_4_8 -> Net-(D7-K2)
- D7 pad 4: OUT_4_9 -> Net-(D7-K3)
- D7 pad 5: OUT_4_10 -> Net-(D7-K4)
- D7 pad 6: OUT_5_1 -> Net-(D7-K5)
- D7 pad 7: OUT_5_2 -> Net-(D7-K6)
- D7 pad 8: OUT_5_3 -> Net-(D7-K7)
- D7 pad 9: OUT_5_4 -> Net-(D7-K8)
- D8 pad 1: OUT_5_5 -> Net-(D8-K1)
- D8 pad 2: OUT_5_6 -> Net-(D8-K2)
- D8 pad 4: OUT_5_7 -> Net-(D8-K3)
- D8 pad 5: OUT_5_8 -> Net-(D8-K4)
- D8 pad 6: OUT_5_9 -> Net-(D8-K5)
- D8 pad 7: OUT_5_10 -> Net-(D8-K6)
- D8 pad 8: unconnected-(D8-K7-Pad8) -> Net-(D8-K7)
- D8 pad 9: unconnected-(D8-K8-Pad9) -> Net-(D8-K8)
- D9 pad 1: OUT_6_1 -> Net-(D9-K1)
- D9 pad 2: OUT_6_2 -> Net-(D9-K2)
- D9 pad 4: OUT_6_3 -> Net-(D9-K3)
- D9 pad 5: OUT_6_4 -> Net-(D9-K4)
- D9 pad 6: OUT_6_5 -> Net-(D9-K5)
- D9 pad 7: OUT_6_6 -> Net-(D9-K6)
- D9 pad 8: OUT_6_7 -> Net-(D9-K7)
- D9 pad 9: OUT_6_8 -> Net-(D9-K8)
- U1 pad 14: Net-(U1-NRST) -> /Core/NRST
- U1 pad 15: unconnected-(U1-PC0-Pad15) -> /BLE/BLE_SPI_CS1
- U1 pad 16: unconnected-(U1-PC1-Pad16) -> /BLE/BLE_SPI_MOSI
- U1 pad 17: unconnected-(U1-PC2_C-Pad17) -> /BLE/BLE_SPI_MISO
- U1 pad 18: unconnected-(U1-PC3_C-Pad18) -> /BLE/BLE_SPI_CS2
- U1 pad 22: unconnected-(U1-PA0-Pad22) -> /BLE/GDO0_1
- U1 pad 23: unconnected-(U1-PA1-Pad23) -> /BLE/GDO2_1
- U1 pad 24: unconnected-(U1-PA2-Pad24) -> /BLE/GDO0_2
- U1 pad 25: unconnected-(U1-PA3-Pad25) -> /BLE/GDO2_2
- U1 pad 28: unconnected-(U1-PA4-Pad28) -> Net-(U1-PA4)
- U1 pad 29: unconnected-(U1-PA5-Pad29) -> Net-(U1-PA5)
- U1 pad 3: unconnected-(U1-PE4-Pad3) -> Net-(U1-PE4)
- U1 pad 30: unconnected-(U1-PA6-Pad30) -> /Core/SPI1_MISO
- U1 pad 31: unconnected-(U1-PA7-Pad31) -> /Core/SPI1_MOSI
- U1 pad 32: unconnected-(U1-PC4-Pad32) -> /Core/AMS330_CS
- U1 pad 33: unconnected-(U1-PC5-Pad33) -> /Core/AMS330_INT1
- U1 pad 34: unconnected-(U1-PB0-Pad34) -> /Core/AMS330_INT2
- U1 pad 35: unconnected-(U1-PB1-Pad35) -> Net-(D4-K)
- U1 pad 40: unconnected-(U1-PE10-Pad40) -> Net-(D27-K)
- U1 pad 41: unconnected-(U1-PE11-Pad41) -> Net-(D28-K)
- U1 pad 43: unconnected-(U1-PE13-Pad43) -> /Core/TMP_ALERT
- U1 pad 44: unconnected-(U1-PE14-Pad44) -> /Core/EN_L10
- U1 pad 45: unconnected-(U1-PE15-Pad45) -> /Core/EN_L9
- U1 pad 46: unconnected-(U1-PB10-Pad46) -> /BLE/BLE_SPI_CLK
- U1 pad 47: unconnected-(U1-PB11-Pad47) -> /Core/EN_L8
- U1 pad 51: unconnected-(U1-PB12-Pad51) -> /Core/EN_L7
- U1 pad 52: unconnected-(U1-PB13-Pad52) -> /Core/EN_L6
- U1 pad 53: unconnected-(U1-PB14-Pad53) -> /USB-PD/D1-
- U1 pad 54: unconnected-(U1-PB15-Pad54) -> /USB-PD/D1+
- U1 pad 55: unconnected-(U1-PD8-Pad55) -> /Core/EN_L5
- U1 pad 56: unconnected-(U1-PD9-Pad56) -> /Core/EN_L4
- U1 pad 57: unconnected-(U1-PD10-Pad57) -> /Core/EN_L3
- U1 pad 58: unconnected-(U1-PD11-Pad58) -> /Core/EN_L2
- U1 pad 59: unconnected-(U1-PD12-Pad59) -> /Core/EN_L1
- U1 pad 60: unconnected-(U1-PD13-Pad60) -> /Core/LE12
- U1 pad 61: unconnected-(U1-PD14-Pad61) -> /Core/D8
- U1 pad 62: unconnected-(U1-PD15-Pad62) -> /Core/D7
- U1 pad 63: unconnected-(U1-PC6-Pad63) -> /Core/D6
- U1 pad 64: unconnected-(U1-PC7-Pad64) -> /Core/D5
- U1 pad 65: unconnected-(U1-PC8-Pad65) -> /Core/D4
- U1 pad 66: unconnected-(U1-PC9-Pad66) -> /Core/D3
- U1 pad 67: unconnected-(U1-PA8-Pad67) -> /Core/D2
- U1 pad 68: unconnected-(U1-PA9-Pad68) -> /Core/D1
- U1 pad 69: unconnected-(U1-PA10-Pad69) -> /Core/_OE
- U1 pad 70: unconnected-(U1-PA11-Pad70) -> /USB-PD/D0-
- U1 pad 71: unconnected-(U1-PA12-Pad71) -> /USB-PD/D0+
- U1 pad 72: unconnected-(U1-PA13-Pad72) -> Net-(U1-PA13)
- U1 pad 76: unconnected-(U1-PA14-Pad76) -> Net-(U1-PA14)
- U1 pad 77: unconnected-(U1-PA15-Pad77) -> /Core/LE0
- U1 pad 78: unconnected-(U1-PC10-Pad78) -> /Core/LE1
- U1 pad 79: unconnected-(U1-PC11-Pad79) -> /Core/LE2
- U1 pad 80: unconnected-(U1-PC12-Pad80) -> /Core/LE3
- U1 pad 81: unconnected-(U1-PD0-Pad81) -> /Core/LE4
- U1 pad 82: unconnected-(U1-PD1-Pad82) -> /Core/LE5
- U1 pad 83: unconnected-(U1-PD2-Pad83) -> /Core/LE6
- U1 pad 84: unconnected-(U1-PD3-Pad84) -> /Core/LE7
- U1 pad 85: unconnected-(U1-PD4-Pad85) -> /Core/LE8
- U1 pad 86: unconnected-(U1-PD5-Pad86) -> /Core/LE9
- U1 pad 87: unconnected-(U1-PD6-Pad87) -> /Core/LE10
- U1 pad 88: unconnected-(U1-PD7-Pad88) -> /Core/LE11
- U1 pad 89: unconnected-(U1-PB3-Pad89) -> /Core/SPI1_SCK
- U1 pad 90: unconnected-(U1-PB4-Pad90) -> /Core/IIS2MDCTR_DRDY
- U1 pad 91: unconnected-(U1-PB5-Pad91) -> /Core/STUSB4500_ALERT
- U1 pad 92: unconnected-(U1-PB6-Pad92) -> /Core/I2C1_SCL
- U1 pad 93: unconnected-(U1-PB7-Pad93) -> /Core/I2C1_SDA
- U10 pad 1: /Multiplexer/_OE -> /Core/_OE
- U10 pad 11: /Multiplexer/LE8 -> /Core/LE1
- U10 pad 12: OUT_6_5 -> Net-(D8-K6)
- U10 pad 13: /Multiplexer/D5 -> /Core/D5
- U10 pad 14: /Multiplexer/D6 -> /Core/D6
- U10 pad 15: OUT_6_6 -> Net-(D8-K5)
- U10 pad 16: OUT_6_7 -> Net-(D8-K3)
- U10 pad 17: /Multiplexer/D7 -> /Core/D7
- U10 pad 18: /Multiplexer/D8 -> /Core/D8
- U10 pad 19: OUT_6_8 -> Net-(D8-K4)
- U10 pad 2: OUT_6_1 -> Net-(D8-K1)
- U10 pad 21: unconnected-(U10-EPAD-Pad21) -> GND
- U10 pad 3: /Multiplexer/D1 -> /Core/D1
- U10 pad 4: /Multiplexer/D2 -> /Core/D2
- U10 pad 5: OUT_6_2 -> Net-(D8-K2)
- U10 pad 6: OUT_6_3 -> Net-(D8-K8)
- U10 pad 7: /Multiplexer/D3 -> /Core/D3
- U10 pad 8: /Multiplexer/D4 -> /Core/D4
- U10 pad 9: OUT_6_4 -> Net-(D8-K7)
- U10 pad V: (no net) -> GND
- U11 pad 1: /Multiplexer/_OE -> /Core/_OE
- U11 pad 11: /Multiplexer/LE9 -> /Core/LE5
- U11 pad 12: OUT_7_3 -> Net-(D9-K6)
- U11 pad 13: /Multiplexer/D5 -> /Core/D5
- U11 pad 14: /Multiplexer/D6 -> /Core/D6
- U11 pad 15: OUT_7_4 -> Net-(D9-K5)
- U11 pad 16: OUT_7_5 -> Net-(D9-K3)
- U11 pad 17: /Multiplexer/D7 -> /Core/D7
- U11 pad 18: /Multiplexer/D8 -> /Core/D8
- U11 pad 19: OUT_7_6 -> Net-(D9-K4)
- U11 pad 2: OUT_6_9 -> Net-(D9-K1)
- U11 pad 21: unconnected-(U11-EPAD-Pad21) -> GND
- U11 pad 3: /Multiplexer/D1 -> /Core/D1
- U11 pad 4: /Multiplexer/D2 -> /Core/D2
- U11 pad 5: OUT_6_10 -> Net-(D9-K2)
- U11 pad 6: OUT_7_1 -> Net-(D9-K8)
- U11 pad 7: /Multiplexer/D3 -> /Core/D3
- U11 pad 8: /Multiplexer/D4 -> /Core/D4
- U11 pad 9: OUT_7_2 -> Net-(D9-K7)
- U11 pad V: (no net) -> GND
- U12 pad 1: /Multiplexer/_OE -> /Core/_OE
- U12 pad 11: /Multiplexer/LE10 -> /Core/LE9
- U12 pad 12: OUT_8_1 -> Net-(D10-K6)
- U12 pad 13: /Multiplexer/D5 -> /Core/D5
- U12 pad 14: /Multiplexer/D6 -> /Core/D6
- U12 pad 15: OUT_8_2 -> Net-(D10-K5)
- U12 pad 16: OUT_8_3 -> Net-(D10-K3)
- U12 pad 17: /Multiplexer/D7 -> /Core/D7
- U12 pad 18: /Multiplexer/D8 -> /Core/D8
- U12 pad 19: OUT_8_4 -> Net-(D10-K4)
- U12 pad 2: OUT_7_7 -> Net-(D10-K1)
- U12 pad 21: unconnected-(U12-EPAD-Pad21) -> GND
- U12 pad 3: /Multiplexer/D1 -> /Core/D1
- U12 pad 4: /Multiplexer/D2 -> /Core/D2
- U12 pad 5: OUT_7_8 -> Net-(D10-K2)
- U12 pad 6: OUT_7_9 -> Net-(D10-K8)
- U12 pad 7: /Multiplexer/D3 -> /Core/D3
- U12 pad 8: /Multiplexer/D4 -> /Core/D4
- U12 pad 9: OUT_7_10 -> Net-(D10-K7)
- U12 pad V: (no net) -> GND
- U13 pad 1: /Multiplexer/_OE -> /Core/_OE
- U13 pad 11: /Multiplexer/LE11 -> /Core/LE2
- U13 pad 12: OUT_8_9 -> Net-(D11-K6)
- U13 pad 13: /Multiplexer/D5 -> /Core/D5
- U13 pad 14: /Multiplexer/D6 -> /Core/D6
- U13 pad 15: OUT_8_10 -> Net-(D11-K5)
- U13 pad 16: OUT_9_9 -> Net-(D11-K3)
- U13 pad 17: /Multiplexer/D7 -> /Core/D7
- U13 pad 18: /Multiplexer/D8 -> /Core/D8
- U13 pad 19: OUT_9_10 -> Net-(D11-K4)
- U13 pad 2: OUT_8_5 -> Net-(D11-K1)
- U13 pad 21: unconnected-(U13-EPAD-Pad21) -> GND
- U13 pad 3: /Multiplexer/D1 -> /Core/D1
- U13 pad 4: /Multiplexer/D2 -> /Core/D2
- U13 pad 5: OUT_8_6 -> Net-(D11-K2)
- U13 pad 6: OUT_8_7 -> Net-(D11-K8)
- U13 pad 7: /Multiplexer/D3 -> /Core/D3
- U13 pad 8: /Multiplexer/D4 -> /Core/D4
- U13 pad 9: OUT_8_8 -> Net-(D11-K7)
- U13 pad V: (no net) -> GND
- U14 pad 1: /Multiplexer/_OE -> /Core/_OE
- U14 pad 11: /Multiplexer/LE12 -> /Core/LE6
- U14 pad 12: OUT_9_5 -> Net-(D12-K6)
- U14 pad 13: /Multiplexer/D5 -> /Core/D5
- U14 pad 14: /Multiplexer/D6 -> /Core/D6
- U14 pad 15: OUT_9_6 -> Net-(D12-K5)
- U14 pad 16: OUT_9_7 -> Net-(D12-K3)
- U14 pad 17: /Multiplexer/D7 -> /Core/D7
- U14 pad 18: /Multiplexer/D8 -> /Core/D8
- U14 pad 19: OUT_9_8 -> Net-(D12-K4)
- U14 pad 2: OUT_9_1 -> Net-(D12-K1)
- U14 pad 21: unconnected-(U14-EPAD-Pad21) -> GND
- U14 pad 3: /Multiplexer/D1 -> /Core/D1
- U14 pad 4: /Multiplexer/D2 -> /Core/D2
- U14 pad 5: OUT_9_2 -> Net-(D12-K2)
- U14 pad 6: OUT_9_3 -> Net-(D12-K8)
- U14 pad 7: /Multiplexer/D3 -> /Core/D3
- U14 pad 8: /Multiplexer/D4 -> /Core/D4
- U14 pad 9: OUT_9_4 -> Net-(D12-K7)
- U14 pad V: (no net) -> GND
- U2 pad 1: /Multiplexer/_OE -> Net-(U1-PA5)
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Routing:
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- added copper zone on In2.Cu, net +3.3V
- added copper zone on B.Cu, net GND
- added copper zone on F.Cu, net GND
- added copper zone on In1.Cu, net GND
- added copper zone on In2.Cu, net Net-(D21-K)
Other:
- board size 102 x 102 mm -> 87.7 x 80.2 mm
- copper layers 2 -> 4
- board text added: "Hij loopd"
- board text added: "mikai was here"
